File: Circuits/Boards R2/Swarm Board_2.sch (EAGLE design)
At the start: 94 parts, among them CON1 ISP(2X3), CON2 MAIN_CONNECTOR, CON3 FTDI_3PIN, CON4 POWERJUMPER, T1 NPN2N2222, T10 TEFT4300, T11 NPN2N2222, T13 NPN2N2222, T14 NPN2N2222, T15 NPN2N2222, T16 NPN2N2222, T17 NPN2N2222, T18 NPN2N2222, T2 NPN2N2222, T3 NPN2N2222, T4 TEFT4300, T5 TEFT4300, T6 TEFT4300, T7 TEFT4300, T8 TEFT4300, T9 TEFT4300, U1 ATMEGA324P, U2 MCP73833

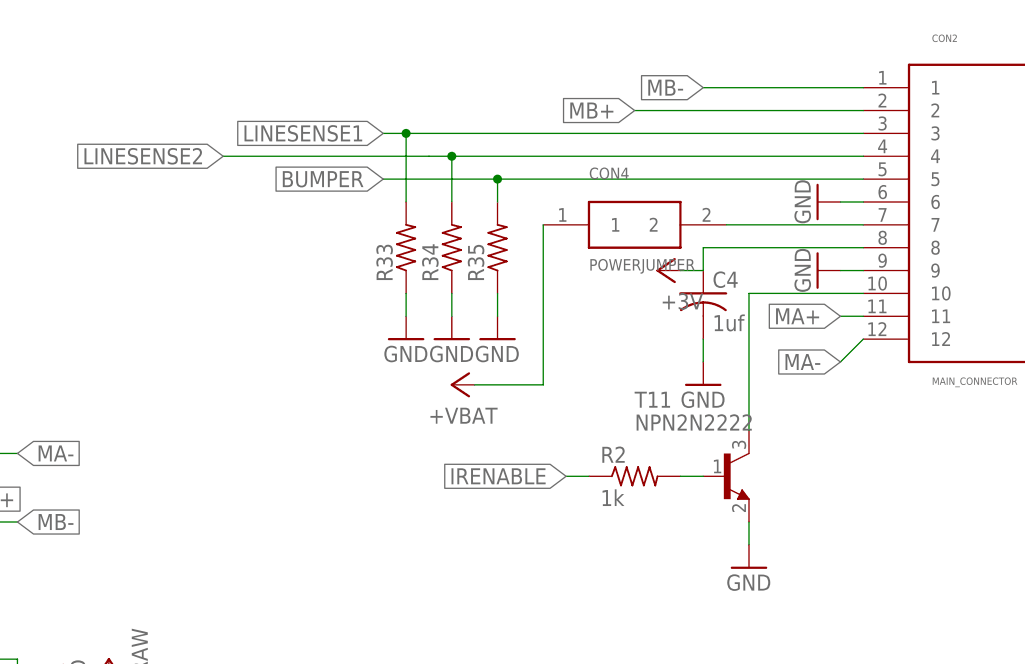
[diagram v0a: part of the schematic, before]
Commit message: updated R2 board
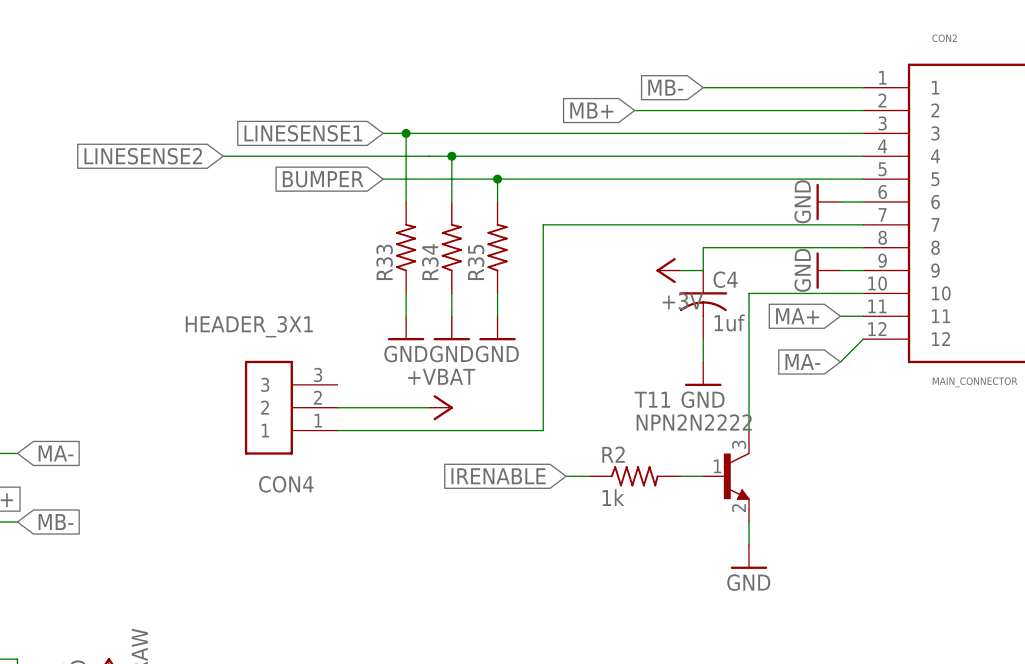
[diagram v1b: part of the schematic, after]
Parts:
- CON4: value POWERJUMPER -> HEADER_3X1; device Mechanical:POWERJUMPER -> Mechanical:HEADER_3X1
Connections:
- net +VBAT: now also CON4.2; no longer CON4.1
- net N$29: now also CON4.1; no longer CON4.2
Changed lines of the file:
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@@
 <?xml version="1.0" encoding="utf-8"?>
 <!DOCTYPE eagle SYSTEM "eagle.dtd">
-<eagle version="6.2">
+<eagle version="6.3">
 <drawing>
 <settings>
@@
 <part name="B1" library="Passive" deviceset="PIEZOBUZZER" device="PTH"/>
 <part name="P+4" library="Supply" deviceset="+3V" device=""/>
-<part name="CON4" library="Mechanical" deviceset="POWERJUMPER" device=""/>
+<part name="CON4" library="Mechanical" deviceset="HEADER_3X1" device=""/>
 <part name="P+16" library="Supply" deviceset="+VBAT" device=""/>
 </parts>
@@
 <instance part="B1" gate="G$1" x="-119.38" y="35.56"/>
 <instance part="P+4" gate="1" x="-71.12" y="7.62" rot="R270"/>
-<instance part="CON4" gate="G$1" x="73.66" y="-109.22"/>
-<instance part="P+16" gate="G$1" x="58.42" y="-127" rot="R90"/>
+<instance part="CON4" gate="G$1" x="38.1" y="-129.54" rot="R180"/>
+<instance part="P+16" gate="G$1" x="53.34" y="-129.54" rot="R270"/>
 </instances>
 <busses>
@@
 </segment>
 <segment>
-<pinref part="CON4" gate="G$1" pin="1"/>
-<wire x1="66.04" y1="-109.22" x2="66.04" y2="-127" width="0.1524" layer="91"/>
-<wire x1="66.04" y1="-127" x2="58.42" y2="-127" width="0.1524" layer="91"/>
+<pinref part="CON4" gate="G$1" pin="2"/>
+<wire x1="43.18" y1="-129.54" x2="53.34" y2="-129.54" width="0.1524" layer="91"/>
 <pinref part="P+16" gate="G$1" pin="+VBAT"/>
 </segment>
@@
 <segment>
 <pinref part="CON2" gate="G$1" pin="7"/>
-<pinref part="CON4" gate="G$1" pin="2"/>
-<wire x1="101.6" y1="-109.22" x2="86.36" y2="-109.22" width="0.1524" layer="91"/>
-</segment>
-</net>
+<wire x1="101.6" y1="-109.22" x2="66.04" y2="-109.22" width="0.1524" layer="91"/>
+<wire x1="66.04" y1="-109.22" x2="66.04" y2="-132.08" width="0.1524" layer="91"/>
+<pinref part="CON4" gate="G$1" pin="1"/>
+<wire x1="66.04" y1="-132.08" x2="43.18" y2="-132.08" width="0.1524" layer="91"/>
+</segment>
+</net>
